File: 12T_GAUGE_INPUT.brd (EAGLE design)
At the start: 71.1 x 63.2 mm, 111 parts, among them J1 MICRO-SD_CARD_SOCKET, P1_WP_PULLUP 10k, P2_WP_PULLUP 10k, P3_WP_PULLUP 10k

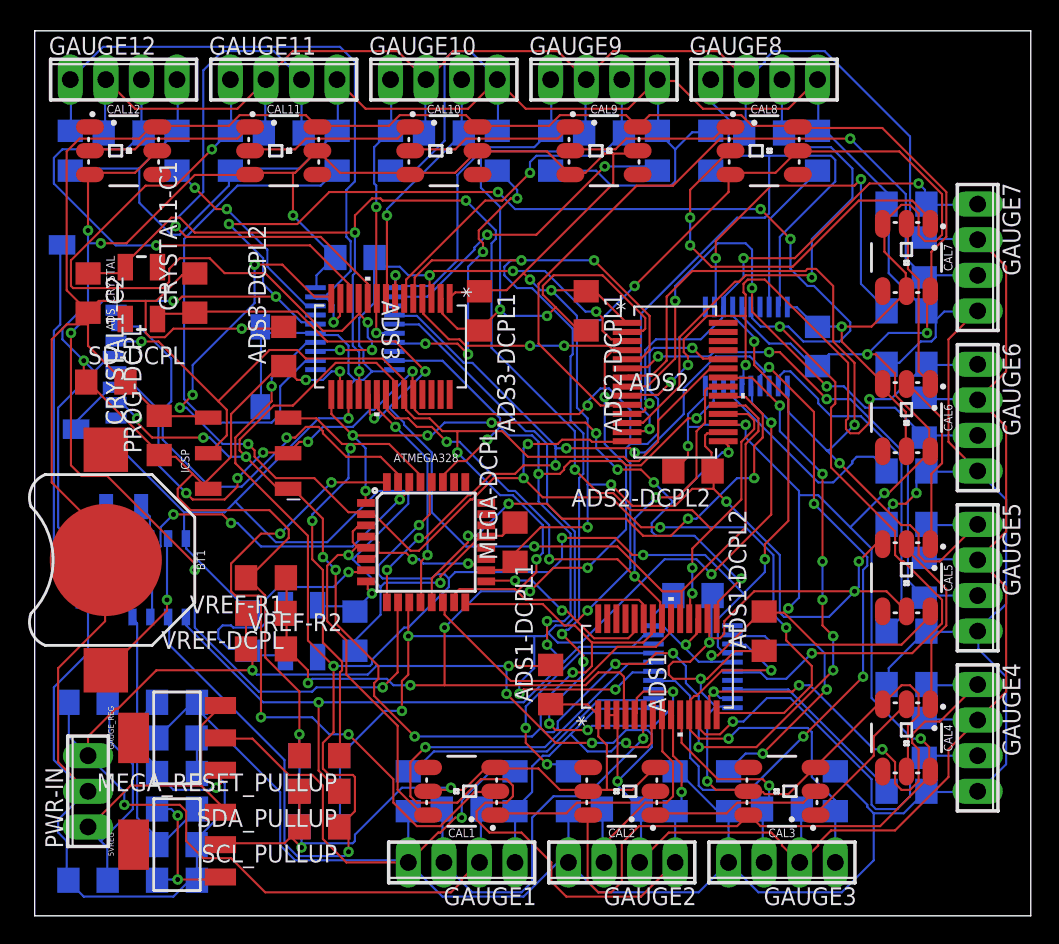
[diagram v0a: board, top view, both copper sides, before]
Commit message: Ground plane
Maybe this will be finished. Maybe it won't.
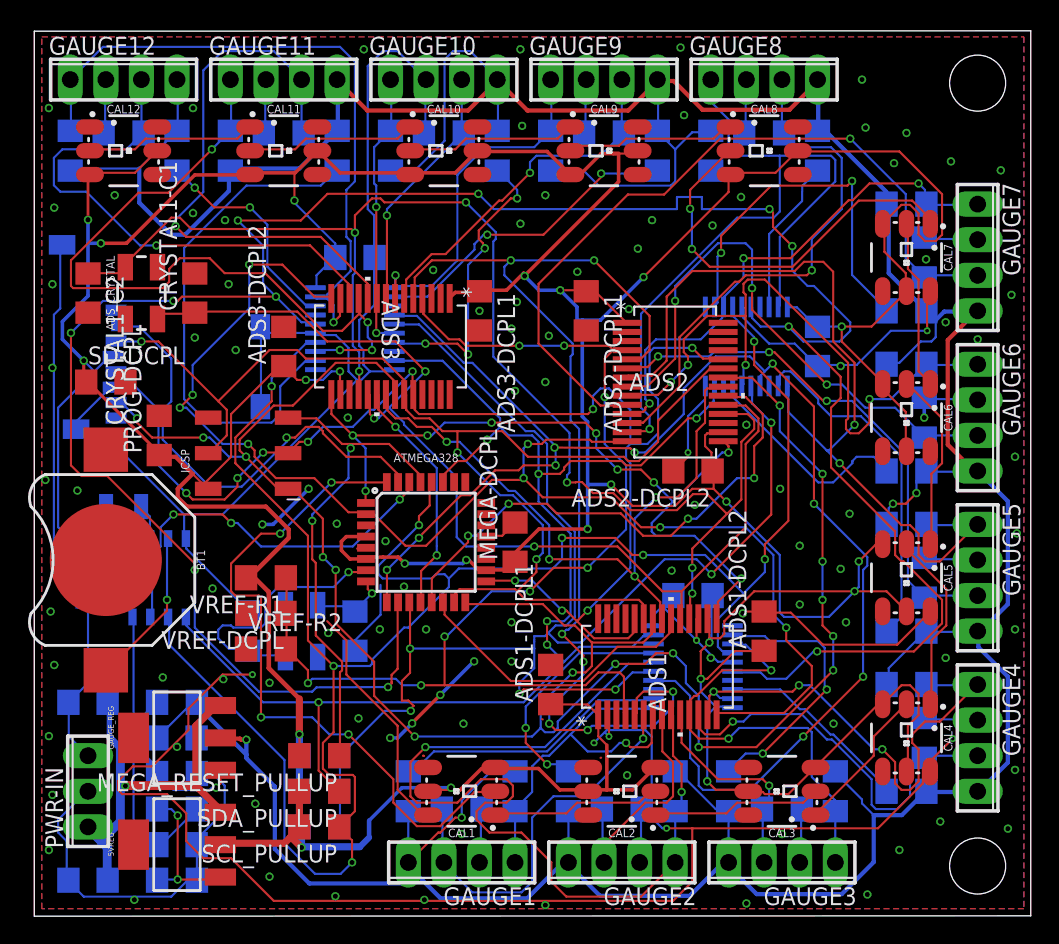
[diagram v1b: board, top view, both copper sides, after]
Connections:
- removed net AGND: ADS1-DCPL1.2, ADS1.2, ADS1.3, ADS2-DCPL1.2, ADS2.2, ADS3-DCPL1.2, ADS3.2, B1-R1.1, B10-R1.1, B11-R1.1, B12-R1.1, B2-R1.1, B3-R1.1, B4-R1.1, B5-R1.1, B6-R1.1, B7-R1.1, B8-R1.1, B9-R1.1, GAUGE1.2, GAUGE10.2, GAUGE11.2, GAUGE12.2, GAUGE2.2, GAUGE3.2, GAUGE4.2, GAUGE5.2, GAUGE6.2, GAUGE7.2, GAUGE8.2, GAUGE9.2, PWR-DCPL-AGND.2, PWR-IN.3, VREF-DCPL.2, VREF-R2.1
- net GND: now also ADS1-DCPL1.2, ADS1.2, ADS1.3, ADS2-DCPL1.2, ADS2.2, ADS3-DCPL1.2, ADS3.2, B1-R1.1, B10-R1.1, B11-R1.1, B12-R1.1, B2-R1.1, B3-R1.1, B4-R1.1, B5-R1.1, B6-R1.1, B7-R1.1, B8-R1.1, B9-R1.1, GAUGE1.2, GAUGE10.2, GAUGE11.2, GAUGE12.2, GAUGE2.2, GAUGE3.2, GAUGE4.2, GAUGE5.2, GAUGE6.2, GAUGE7.2, GAUGE8.2, GAUGE9.2, PWR-DCPL-AGND.2, PWR-IN.3, VREF-DCPL.2, VREF-R2.1
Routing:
- net AGND: track 346.7 -> 0.00 mm, vias 8 -> 0
- net GND: track 555.1 -> 398.1 mm, vias 16 -> 111
- net V+: track 332.1 -> 320.4 mm, vias 3 -> 4
- net +12V: track 34.3 -> 30.0 mm, vias 0 -> 1
- net XTAL2: track 95.5 -> 98.0 mm
- net SCL: track 148.6 -> 150.4 mm
- net AINCOM: track 79.1 -> 77.4 mm
- net POT_SELECT_1: track 176.7 -> 178.3 mm
- net WP: track 104.5 -> 105.7 mm
- net B8+: track 38.5 -> 37.5 mm
- net P3B3: track 14.6 -> 15.6 mm
- net B5-_P2W0: track 59.9 -> 60.9 mm
- net B4+: track 29.2 -> 28.2 mm
- net POT_SELECT_0: track 105.3 -> 106.0 mm
- net B8-_P2W3: track 54.0 -> 54.7 mm
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- added copper zone on layer 1, net GND
- added copper zone on layer 16, net GND
